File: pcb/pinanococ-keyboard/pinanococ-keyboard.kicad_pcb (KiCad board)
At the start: 2 copper layers, 146 x 140.8 mm, 71 parts, among them J1 AudioJack4, SW1 SW_Push, SW10 SW_Push, SW11 SW_Push, SW12 SW_Push, SW14 SW_Push_Dual_x2, SW15 SW_Push, SW16 SW_Push, SW17 SW_Push, SW18 SW_Push, SW2 SW_Push, SW20 SW_Push_Dual_x2, SW21 SW_Push, SW22 SW_Push, SW23 SW_Push, SW24 SW_Push, SW26 SW_Push_Dual_x2, SW27 SW_Push, SW28 SW_Push, SW29 SW_Push, SW3 SW_Push, SW30 SW_Push, SW32 SW_Push_Dual_x2, SW33 SW_Push, SW34 SW_Push, SW35 SW_Push, SW36 SW_Push, SW37 SW_Push, SW38 Rotary_Encoder_Switch, SW4 SW_Push, SW5 SW_Push, SW6 SW_Push, SW8 SW_Push, SW9 SW_Push, U1 Pico

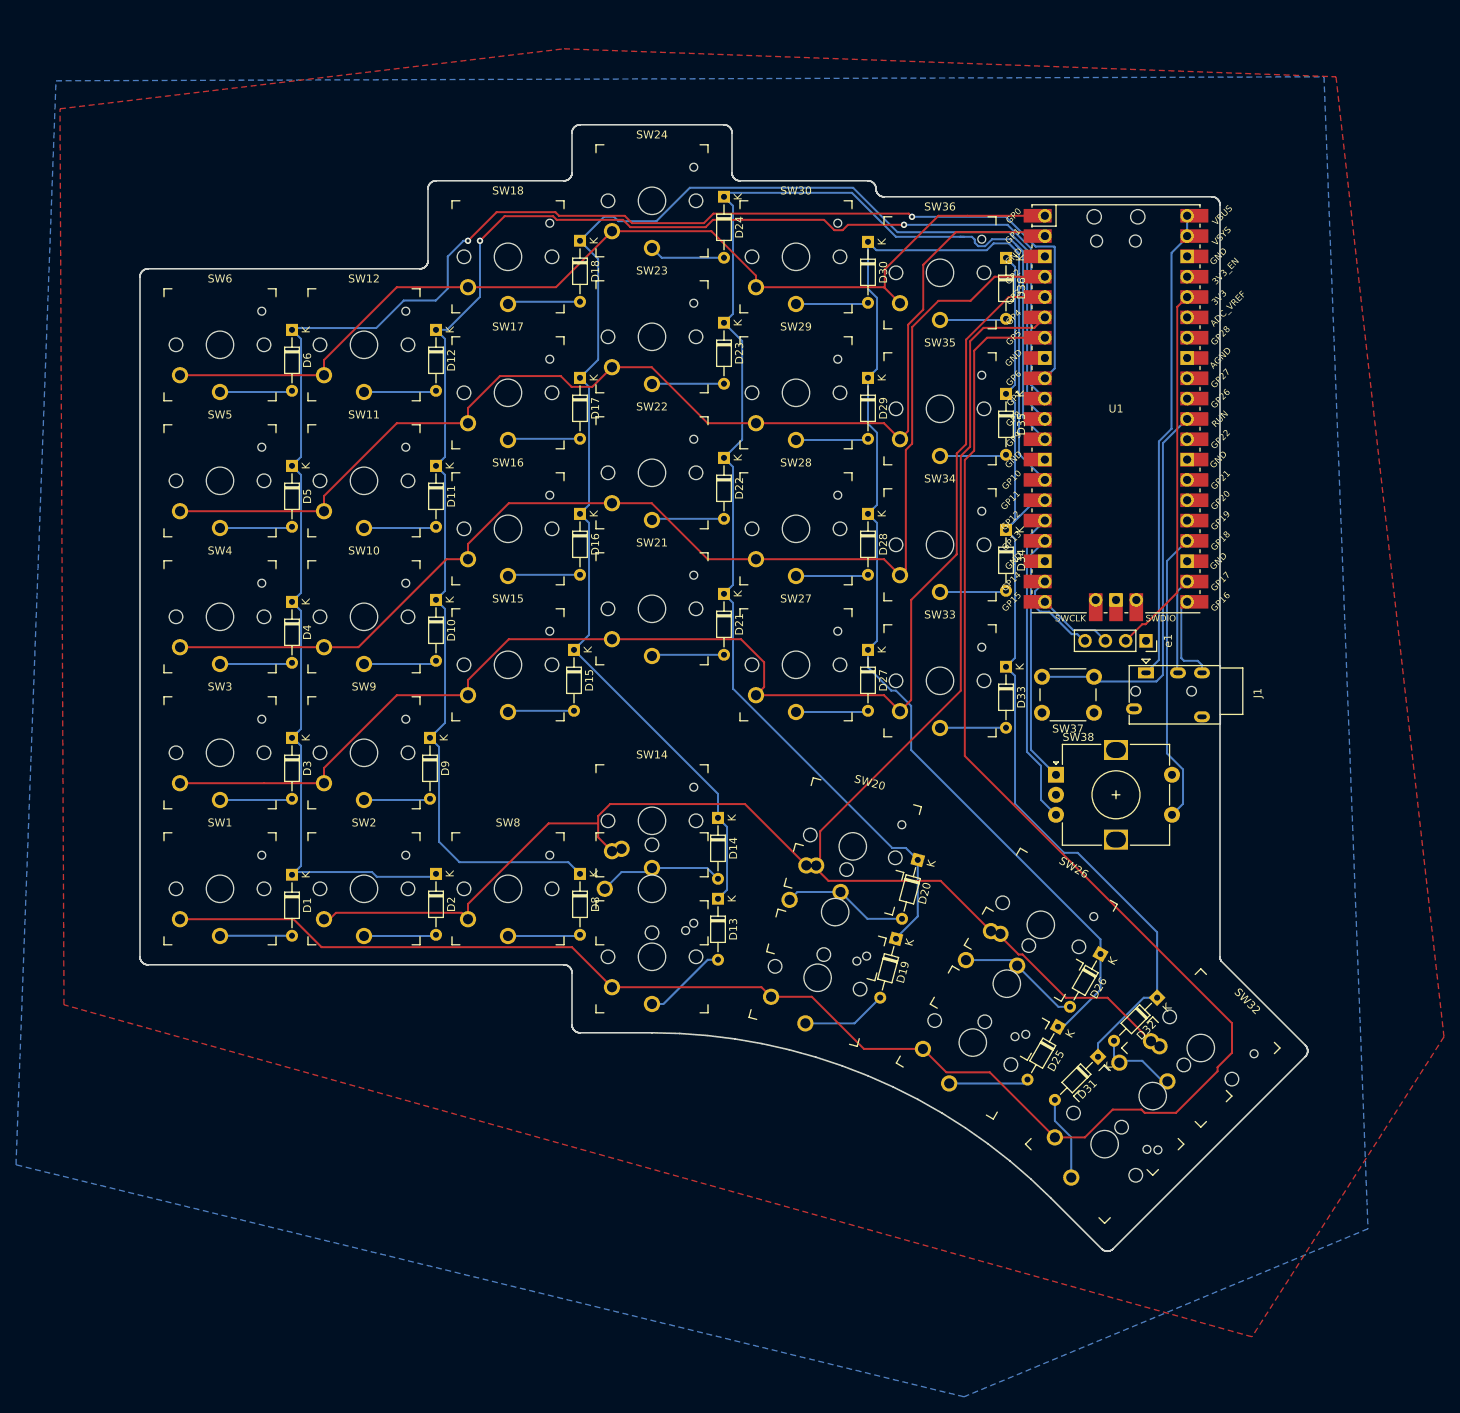
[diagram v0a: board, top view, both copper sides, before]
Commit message: inital switch pcb layout
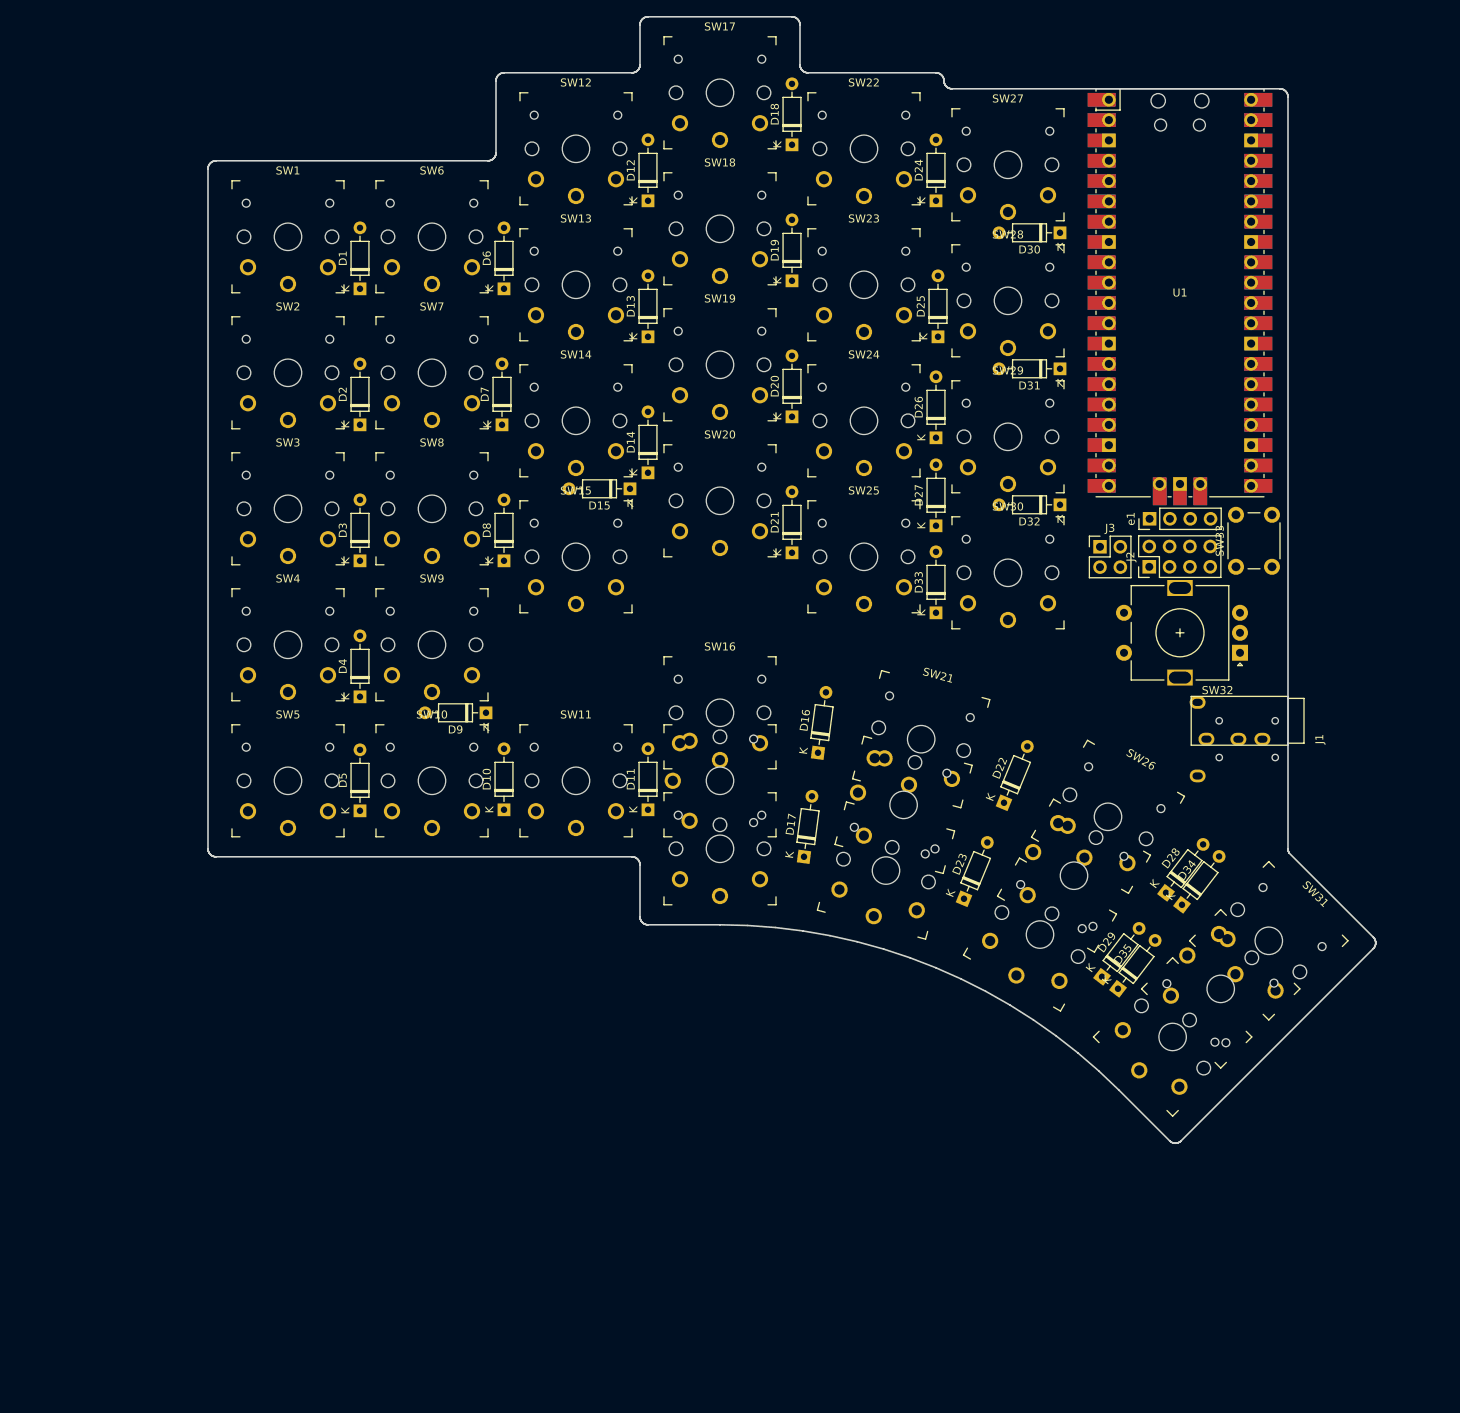
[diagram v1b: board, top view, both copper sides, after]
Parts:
- removed D36: D_ALT, Diode_THT:D_DO-34_SOD68_P7.62mm_Horizontal
- removed SW34, SW35, SW36: SW_Push, keyswitches:SW_PG1350
- removed SW37: SW_Push, Button_Switch_THT:SW_PUSH_6mm
- removed SW38: Rotary_Encoder_Switch, Rotary_Encoder:RotaryEncoder_Alps_EC12E-Switch_Vertical_H20mm
- added D7: D_ALT, Diode_THT:D_DO-35_SOD27_P7.62mm_Horizontal, F.Cu at (59.2, 75.0)
- added J2: Conn_02x04_Top_Bottom, Connector_PinHeader_2.54mm:PinHeader_2x04_P2.54mm_Vertical, F.Cu at (140.2, 92.8)
- added J3: Conn_02x02_Top_Bottom, Connector_PinHeader_2.54mm:PinHeader_2x02_P2.54mm_Vertical, F.Cu at (134.0, 90.2)
- added SW13: SW_Push, keyswitches:SW_PG1350_reversible, F.Cu at (68.5, 57.5)
- added SW19: SW_Push, keyswitches:SW_PG1350_reversible, F.Cu at (86.5, 67.5)
- added SW25: SW_Push, keyswitches:SW_PG1350_reversible, F.Cu at (104.5, 91.5)
- added SW31: SW_Push_Dual_x2, footprints:SW_PG1350_reversible_double_rotatable, F.Cu at (155.1, 139.5)
- added SW7: SW_Push, keyswitches:SW_PG1350_reversible, F.Cu at (50.5, 68.5)
- D1, D10, D11, D12, D13, D14, D15, D16, D17, D18, D19, D2, D20, D21, D22, D23, D24, D25, D26, D27, D28, D29, D3, D30, D31, D32, D33, D34, D35, D4, D5, D6, D8, D9: footprint Diode_THT:D_DO-34_SOD68_P7.62mm_Horizontal -> Diode_THT:D_DO-35_SOD27_P7.62mm_Horizontal
- J1: footprint Connector_Audio:Jack_3.5mm_PJ320E_Horizontal -> footprints:TRRS-PJ-320A_reversable
- SW1, SW10, SW11, SW12, SW15, SW17, SW18, SW2, SW22, SW23, SW24, SW27, SW28, SW29, SW3, SW30, SW4, SW5, SW6, SW8, SW9: footprint keyswitches:SW_PG1350 -> keyswitches:SW_PG1350_reversible
- SW14, SW20: value SW_Push_Dual_x2 -> SW_Push; footprint keyswitches:SW_PG1350_double_rotate -> keyswitches:SW_PG1350_reversible
- SW16, SW21: value SW_Push -> SW_Push_Dual_x2; footprint keyswitches:SW_PG1350 -> footprints:SW_PG1350_reversible_double_rotatable
- SW26: footprint keyswitches:SW_PG1350_double_rotate -> footprints:SW_PG1350_reversible_double_rotatable
- SW32: value SW_Push_Dual_x2 -> Rotary_Encoder_Switch; footprint keyswitches:SW_PG1350_double_rotate -> Rotary_Encoder:RotaryEncoder_Alps_EC11E-Switch_Vertical_H20mm
- SW33: footprint keyswitches:SW_PG1350 -> Button_Switch_THT:SW_PUSH_6mm
- U1: footprint MCU_RaspberryPi_and_Boards:RPi_Pico_SMD_TH -> footprints:RPi_Pico_SMD_TH_flipable
- e1: footprint Connector_PinSocket_2.54mm:PinSocket_1x04_P2.54mm_Vertical -> Connector_PinHeader_2.54mm:PinHeader_1x04_P2.54mm_Vertical
- moved D25 87.5 mm to (113.8, 64.0), turned to 90 degrees
- moved D31 86.1 mm to (129.0, 68.0), turned to 180 degrees
- moved D19 83.3 mm to (95.5, 57.0), turned to 90 degrees
- moved SW1 81.9 mm to (32.5, 51.5)
- moved D29 80.4 mm to (134.2, 144.0), turned to 52.5 degrees
- moved D23 78.0 mm to (117.0, 134.2), turned to 67.5 degrees
- moved D35 75.7 mm to (136.2, 145.5), turned to 52.5 degrees
- moved D1 73.7 mm to (41.5, 58.0), turned to 90 degrees
- moved D13 70.8 mm to (77.5, 64.0), turned to 90 degrees
- moved SW27 67.9 mm to (122.5, 42.5)
- moved D26 67.7 mm to (113.5, 76.6), turned to 90 degrees
- moved D17 66.1 mm to (97.0, 129.0), turned to 82.5 degrees
- moved SW2 65.2 mm to (32.5, 68.5)
- moved D32 62.8 mm to (129.0, 85.0), turned to 180 degrees
- moved D28 60.3 mm to (142.2, 133.5), turned to 52.5 degrees
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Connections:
- D12 pad 1: COL_1 -> COL_2
- D18 pad 1: COL_2 -> COL_3
- D24 pad 1: COL_3 -> COL_4
- D30 pad 1: COL_4 -> COL_5
- D6 pad 1: COL_0 -> COL_1
- SW1 pad 2: ROW_0 -> ROW_5
- SW10 pad 2: ROW_3 -> ROW_1
- SW11 pad 2: ROW_4 -> ROW_0
- SW14 pad 2: ROW_1 -> ROW_3
- SW16 pad 2: ROW_3 -> ROW_1
- SW17 pad 1: Net-(D17-Pad2) -> Net-(D18-Pad2)
- SW17 pad 2: ROW_4 -> ROW_5
- SW18 pad 1: Net-(D18-Pad2) -> Net-(D19-Pad2)
- SW18 pad 2: ROW_5 -> ROW_4
- SW2 pad 2: ROW_1 -> ROW_4
- SW20 pad 1: Net-(D20-Pad2) -> Net-(D21-Pad2)
- SW20 pad 2: ROW_1 -> ROW_2
- SW21 pad 1: Net-(D21-Pad2) -> Net-(D22-Pad2)
- SW21 pad 2: ROW_2 -> ROW_1
- SW22 pad 1: Net-(D22-Pad2) -> Net-(D24-Pad2)
- SW22 pad 2: ROW_3 -> ROW_5
- SW23 pad 1: Net-(D23-Pad2) -> Net-(D25-Pad2)
- SW24 pad 1: Net-(D24-Pad2) -> Net-(D26-Pad2)
- SW24 pad 2: ROW_5 -> ROW_3
- SW26 pad 1: Net-(D26-Pad2) -> Net-(D28-Pad2)
- SW26 pad 3: Net-(D25-Pad2) -> Net-(D29-Pad2)
- SW27 pad 1: Net-(D27-Pad2) -> Net-(D30-Pad2)
- SW27 pad 2: ROW_2 -> ROW_5
- SW28 pad 1: Net-(D28-Pad2) -> Net-(D31-Pad2)
- SW28 pad 2: ROW_3 -> ROW_4
- SW29 pad 1: Net-(D29-Pad2) -> Net-(D32-Pad2)
- SW29 pad 2: ROW_4 -> ROW_3
- SW3 pad 2: ROW_2 -> ROW_3
- SW30 pad 1: Net-(D30-Pad2) -> Net-(D33-Pad2)
- SW30 pad 2: ROW_5 -> ROW_2
- SW33 pad 1: Net-(D33-Pad2) -> GND
- SW33 pad 2: ROW_2 -> Reset
- SW4 pad 2: ROW_3 -> ROW_2
- SW5 pad 2: ROW_4 -> ROW_1
- SW8 pad 2: ROW_1 -> ROW_3
- U1 pad 1: ROW_5 -> VBUS
- U1 pad 10: COL_1 -> ROW_3
- U1 pad 11: COL_2 -> Net-(J3-Pad2)
- U1 pad 12: COL_3 -> ROW_2
- U1 pad 14: COL_4 -> ROW_1
- U1 pad 15: COL_5 -> ROW_0
- U1 pad 16: ROT_B -> UART_TX
- U1 pad 17: ROT_A -> UART_RX
- U1 pad 19: I2C_SDA -> I2C_SCL_SDA
- U1 pad 2: ROW_4 -> VBUS
- U1 pad 20: I2C_SCL -> I2C_SDA_SCL
- U1 pad 21: UART_TX -> ROT_A
- U1 pad 22: UART_RX -> ROT_B
- U1 pad 24: ROT_SW -> UART_TX
- U1 pad 25: Net-(U1-Pad25) -> UART_RX
- U1 pad 26: Net-(U1-Pad26) -> COL_0
- U1 pad 27: Net-(U1-Pad27) -> COL_1
- U1 pad 29: Net-(U1-Pad29) -> COL_2
- U1 pad 30: Reset -> Net-(J3-Pad1)
- U1 pad 31: Net-(U1-Pad31) -> COL_3
- U1 pad 32: Net-(U1-Pad32) -> COL_4
- U1 pad 33: Net-(U1-Pad33) -> GND
- U1 pad 34: Net-(U1-Pad34) -> COL_5
- U1 pad 4: ROW_3 -> Net-(U1-Pad4)
- U1 pad 5: ROW_2 -> +3V3
- U1 pad 6: ROW_1 -> Net-(U1-Pad6)
- U1 pad 7: ROW_0 -> ROW_5
- U1 pad 9: COL_0 -> ROW_4
- e1 pad 1: GND -> Net-(J2-Pad2)
- e1 pad 2: +3V3 -> Net-(J2-Pad4)
- e1 pad 3: I2C_SCL -> Net-(J2-Pad6)
- e1 pad 4: I2C_SDA -> Net-(J2-Pad8)
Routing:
- net ROW_0: track 259.4 -> 0.00 mm
- net ROW_1: track 215.4 -> 0.00 mm
- net COL_0: track 214.4 -> 0.00 mm, vias 2 -> 0
- net COL_1: track 193.7 -> 0.00 mm, vias 2 -> 0
- net COL_2: track 179.0 -> 0.00 mm
- net COL_3: track 177.3 -> 0.00 mm
- net ROW_2: track 169.2 -> 0.00 mm
- net COL_4: track 165.9 -> 0.00 mm
- net ROW_3: track 153.1 -> 0.00 mm
- net ROW_4: track 144.6 -> 0.00 mm
- net ROW_5: track 128.2 -> 0.00 mm
- net COL_5: track 121.9 -> 0.00 mm
- net VBUS: track 59.3 -> 0.00 mm
- net Reset: track 48.9 -> 0.00 mm
- net +3V3: track 46.4 -> 0.00 mm
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- removed copper zone on B.Cu, net GND
- removed copper zone on F.Cu, net GND
